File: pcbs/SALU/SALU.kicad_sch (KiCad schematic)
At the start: 0 parts

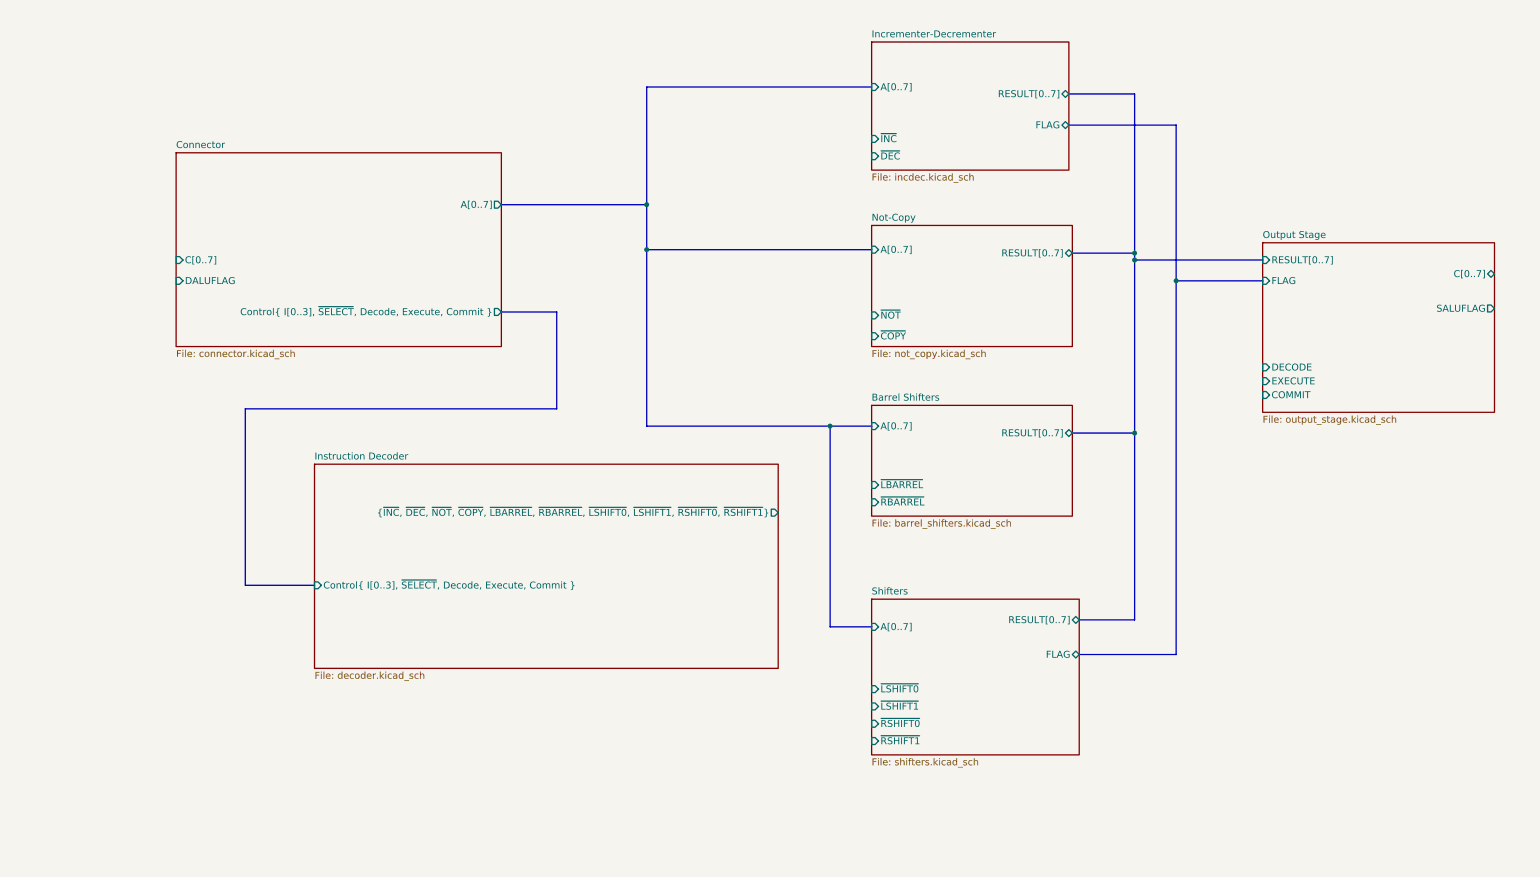
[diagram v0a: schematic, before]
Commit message: Routing
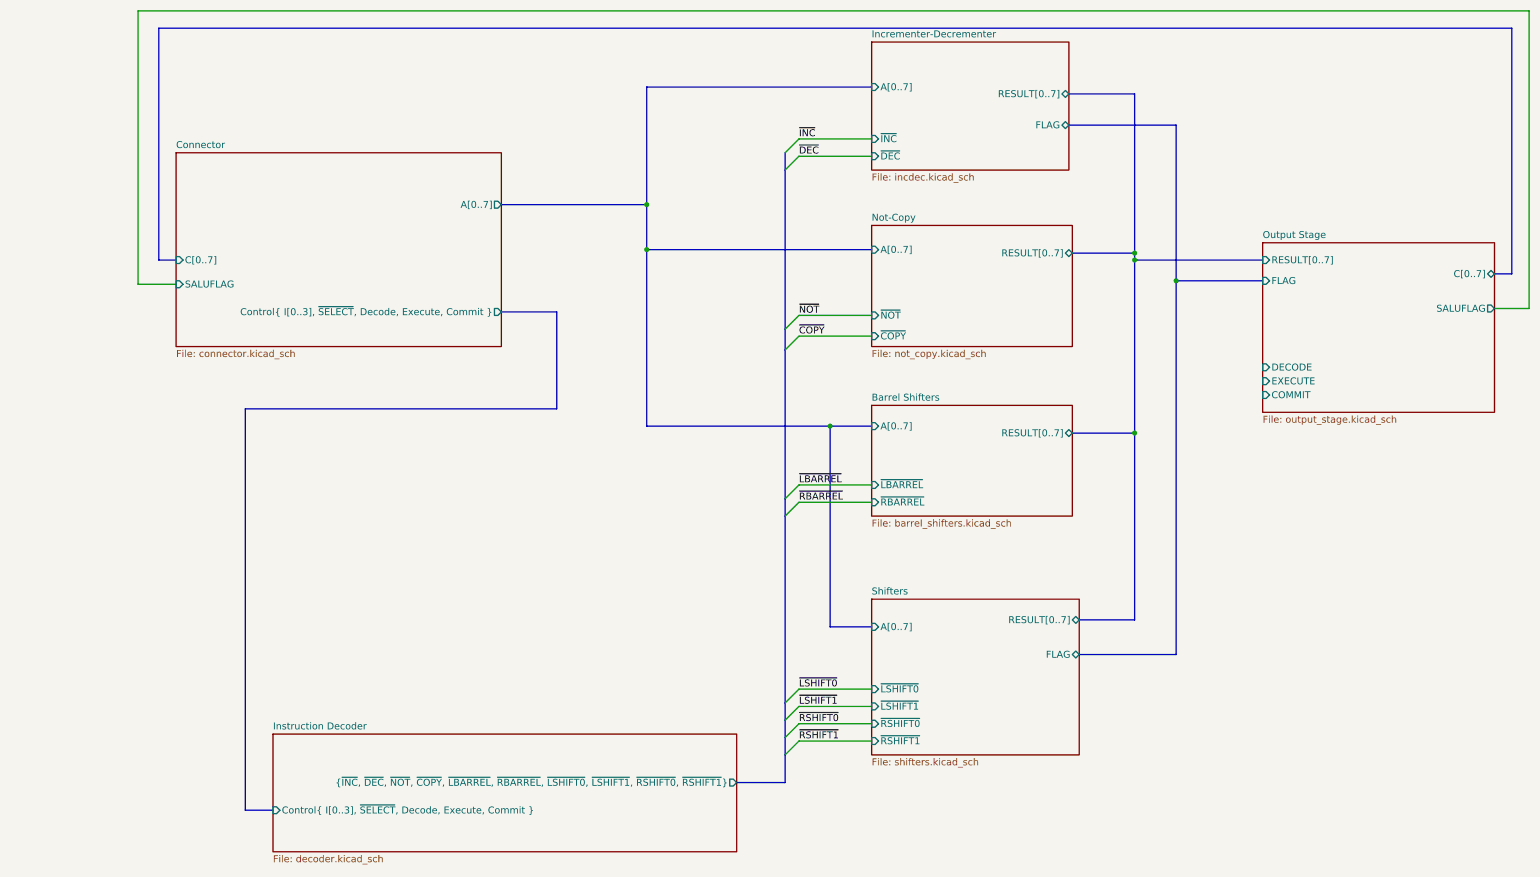
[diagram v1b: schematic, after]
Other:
- sheet Connector ports: added SALUFLAG; removed DALUFLAG
